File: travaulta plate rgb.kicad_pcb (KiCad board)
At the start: 2 copper layers, 210.7 x 77.4 mm, 55 parts

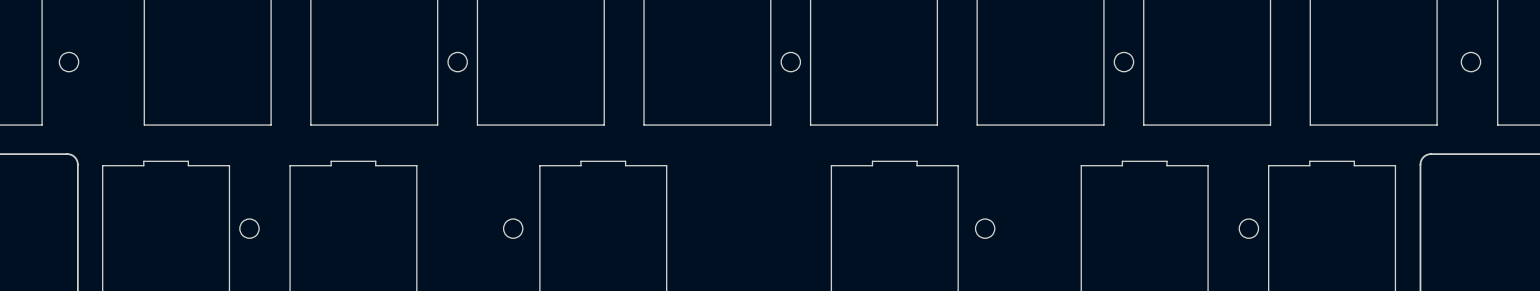
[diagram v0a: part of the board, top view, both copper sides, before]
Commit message: fresh gerbers
deleted old plate gerbers, need new export
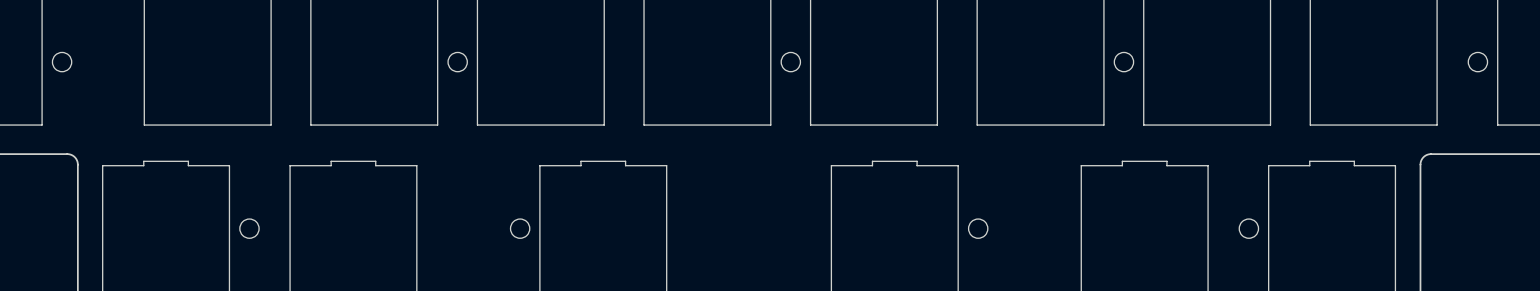
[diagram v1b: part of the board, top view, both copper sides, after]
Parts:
- moved H16 0.79 mm to (175.4, 114.3)
- moved H15 0.79 mm to (123.0, 114.3)
- moved H9 0.79 mm to (70.6, 95.2)
- moved H13 0.79 mm to (232.6, 95.2)
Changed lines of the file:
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@@
   )
   (footprint "cipulot_parts:HOLE_M2" (layer "F.Cu")
-    (at 71.4375 95.25)
+    (at 70.64375 95.25)
     (property "Sheetfile" "mounting holes.kicad_sch")
     (property "Sheetname" "mounting holes")
@@
   )
   (footprint "cipulot_parts:HOLE_M2" (layer "F.Cu")
-    (at 231.775 95.25)
+    (at 232.56875 95.25)
     (property "Sheetfile" "mounting holes.kicad_sch")
     (property "Sheetname" "mounting holes")
@@
   )
   (footprint "cipulot_parts:HOLE_M2" (layer "F.Cu")
-    (at 122.2375 114.3)
+    (at 123.03125 114.3)
     (property "Sheetfile" "mounting holes.kicad_sch")
     (property "Sheetname" "mounting holes")
@@
   )
   (footprint "cipulot_parts:HOLE_M2" (layer "F.Cu")
-    (at 176.2125 114.3)
-    (property "Sheetfile" "mounting holes.kicad_sch")
-    (property "Sheetname" "mounting holes")
+    (at 175.41875 114.3)
+    (property "Sheetfile" "mounting holes.kicad_sch")
+    (property "Sheetname" "mounting holes")

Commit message: pcb clean up, fresh gerbers
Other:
- board text added: "JLCJLCJLCJLC"
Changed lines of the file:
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@@
   (gr_circle (center 63.5 50.574999) (end 64.65 50.574999)
     (stroke (width 0.2) (type solid)) (fill none) (layer "Edge.Cuts"))
+  (gr_text "JLCJLCJLCJLC" (at 249.2375 76.2 -90) (layer "B.SilkS")
+    (effects (font (size 1 1) (thickness 0.15)))
+  )
   (gr_text "RGB Plate" (at 247.65 76.2 270) (layer "F.SilkS")
     (effects (font (size 0.8 0.8) (thickness 0.15)))
